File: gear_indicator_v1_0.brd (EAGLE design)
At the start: 55.5 x 63.5 mm, 30 parts, among them IC1 NE555, IC2 74ALS08N, IC3 74ALS04N, IC4 7805TV, T1 2N3904, T2 2N3904, T3 2N3904

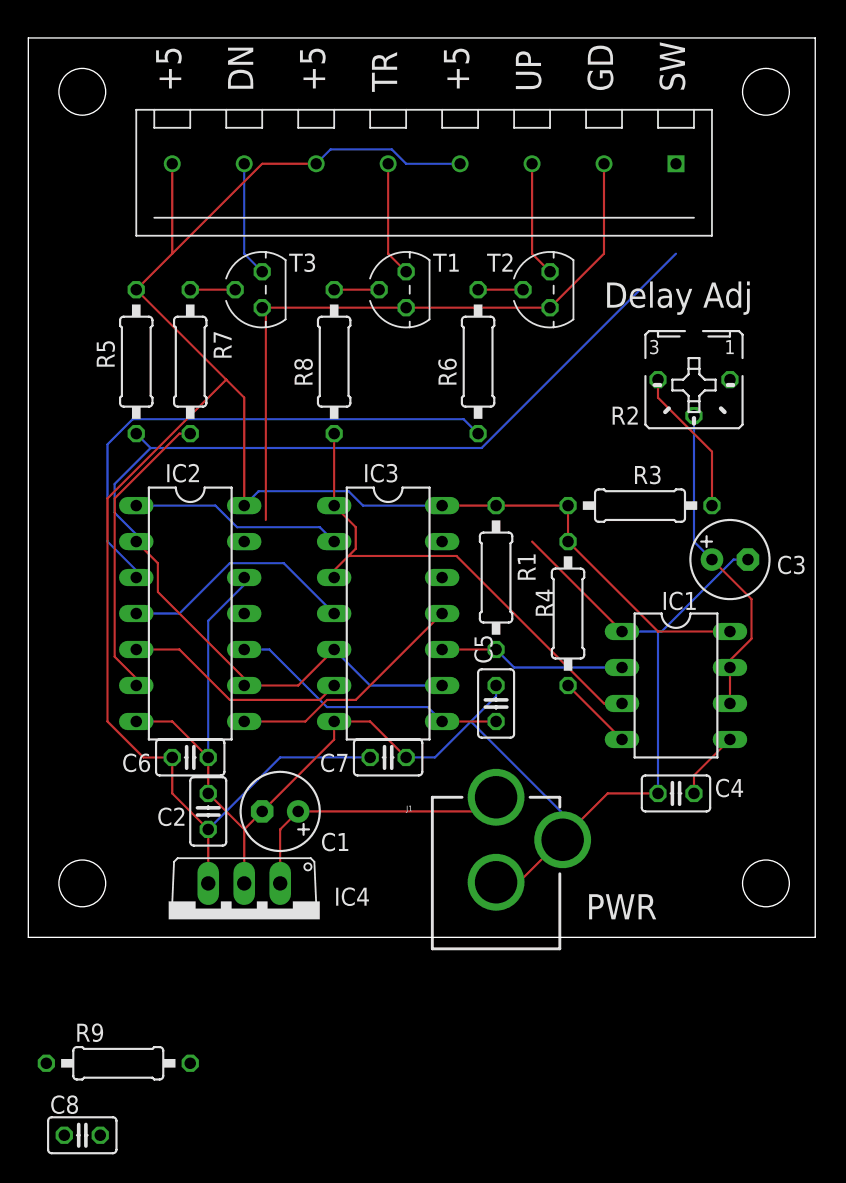
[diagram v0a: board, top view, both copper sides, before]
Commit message: layout tweaks
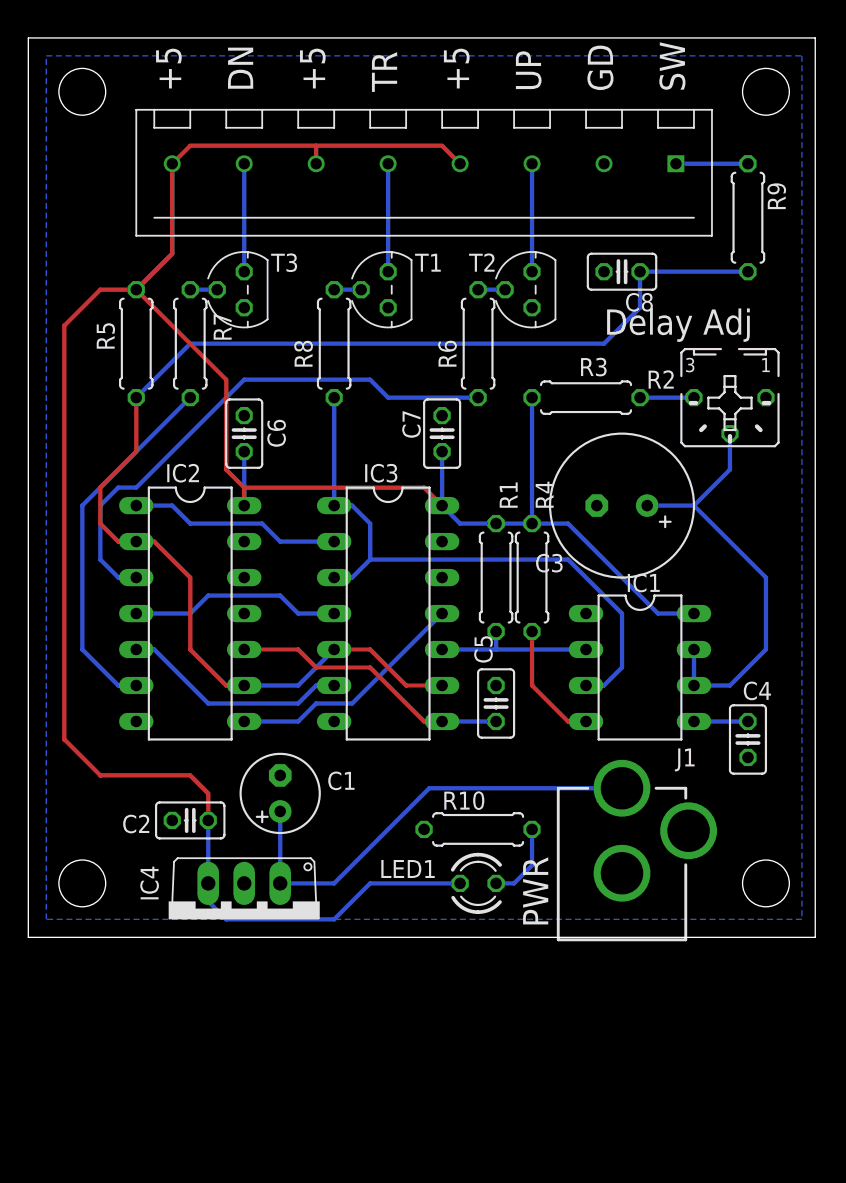
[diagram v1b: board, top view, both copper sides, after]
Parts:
- added LED1: Power, dp_devices:LED-3MM
- added R10: 220, resistor:0207/7
- C3: device rcl:E2,5-6 -> rcl:E3,5-10
- R1, R3, R4, R5, R6, R7, R8, R9: device resistor:0207/10 -> resistor:0207/7
- moved R9 74.4 mm to (50.8, 50.8), turned to 270 degrees
- moved C8 71.9 mm to (41.9, 47.0), turned to 180 degrees
- moved C7 23.2 mm to (29.2, 35.6), turned to 90 degrees
- moved C6 23.2 mm to (15.2, 35.6), turned to 90 degrees
- moved J1 8.91 mm to (41.9, -3.17)
- moved C3 8.52 mm to (41.9, 30.5), turned to 180 degrees
- moved R3 8.52 mm to (39.4, 38.1)
- moved C4 6.35 mm to (50.8, 14.0), turned to 270 degrees
- moved R4 3.59 mm to (35.6, 25.4)
- moved IC1 2.84 mm to (43.2, 19.1)
- moved R2 2.84 mm to (49.5, 38.1)
- moved C2 1.42 mm to (11.4, 8.26), turned to 180 degrees
- moved T1 1.27 mm to (25.4, 45.7)
- moved T3 1.27 mm to (15.2, 45.7)
- moved C1 1.27 mm to (17.8, 10.2), turned to 90 degrees
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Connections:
- new net N$16: LED1.K, R10.2
- net GND: now also R10.1
- net VCC: now also LED1.A
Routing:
- net GND: track 158.2 -> 0.00 mm
- net VCC: track 149.1 -> 186.9 mm
- net N$12: track 20.1 -> 32.0 mm
- net SWITCH: track 81.9 -> 92.2 mm
- net N$2: track 22.6 -> 30.4 mm
- net OUT: track 35.0 -> 42.5 mm
- net N$1: track 10.5 -> 3.81 mm
- net N$16: track 0.00 -> 5.61 mm
- net N$17: track 0.00 -> 5.08 mm
- net N$9: track 21.1 -> 25.8 mm
- net N$3: track 5.39 -> 8.67 mm
- net N$6: track 16.9 -> 15.0 mm
- net TRG: track 13.2 -> 11.4 mm
- net N$13: track 3.18 -> 1.91 mm
- net N$10: track 3.18 -> 1.91 mm
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- added copper zone on layer 16, net GND
